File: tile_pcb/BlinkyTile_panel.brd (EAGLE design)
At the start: 220.1 x 170 mm, 210 parts

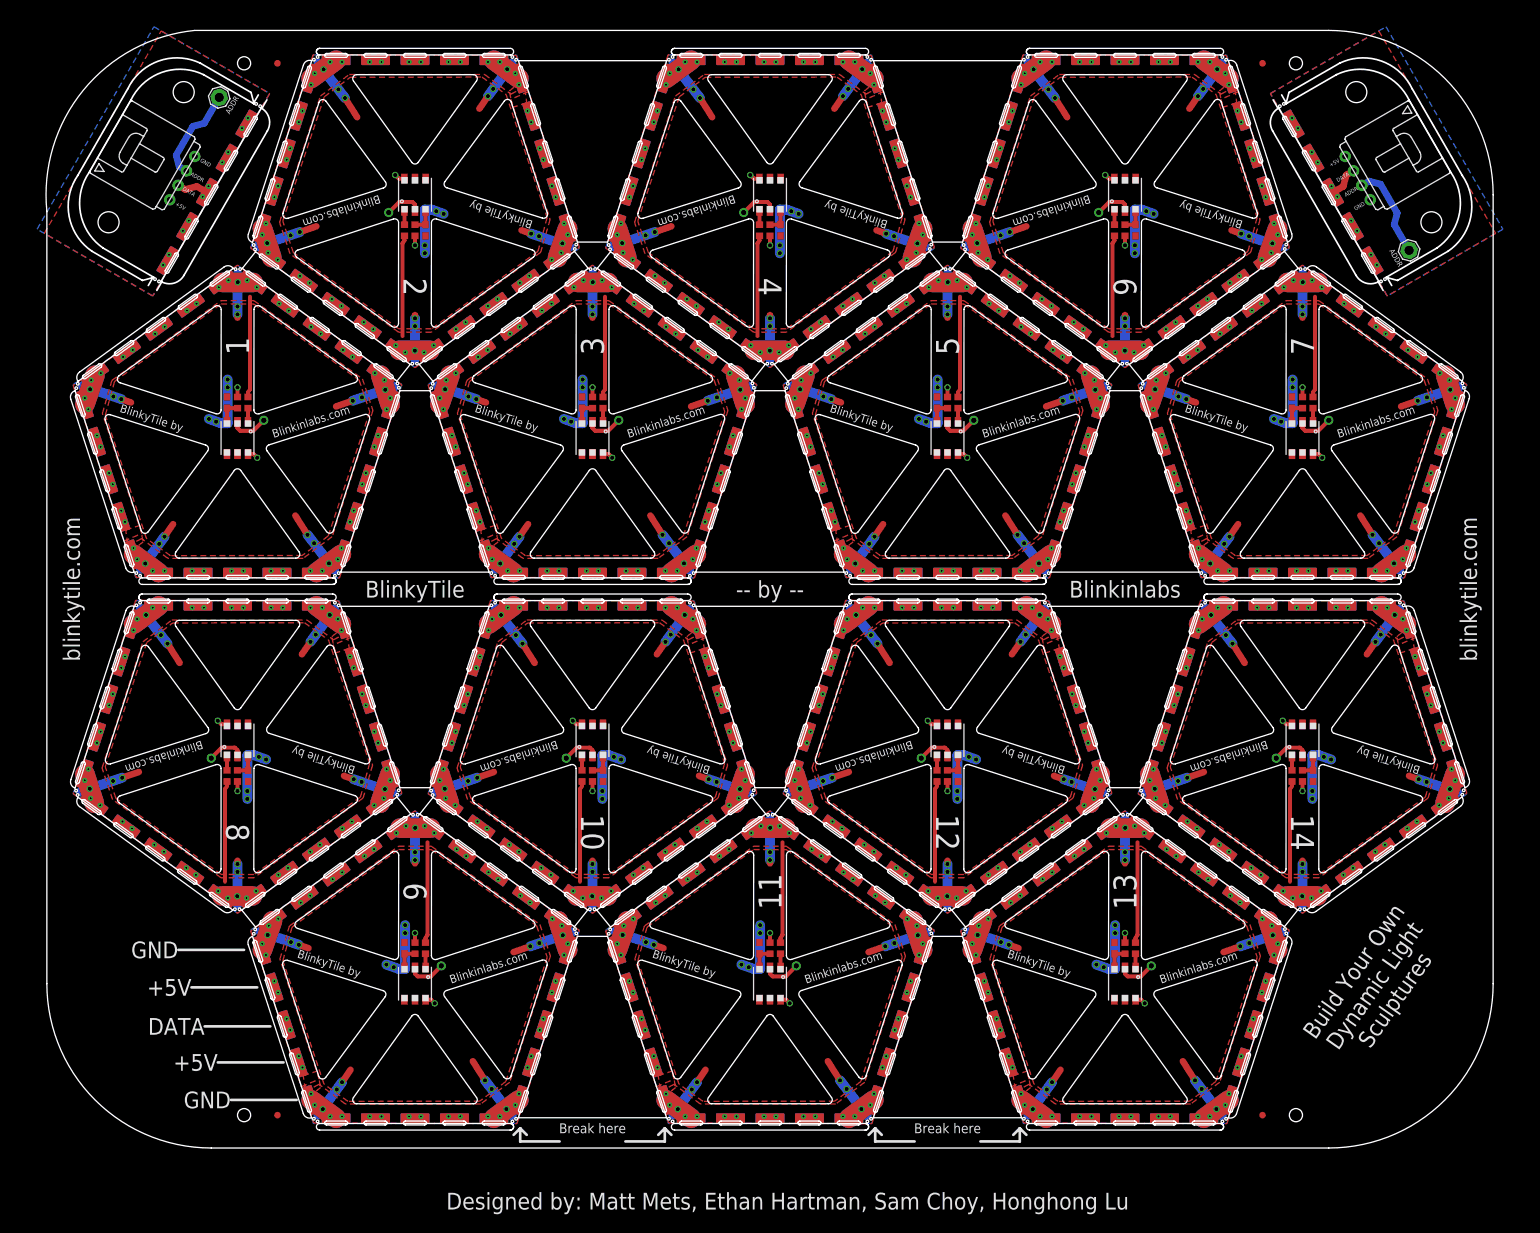
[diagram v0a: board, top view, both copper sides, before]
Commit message: Rev M panel from Sam
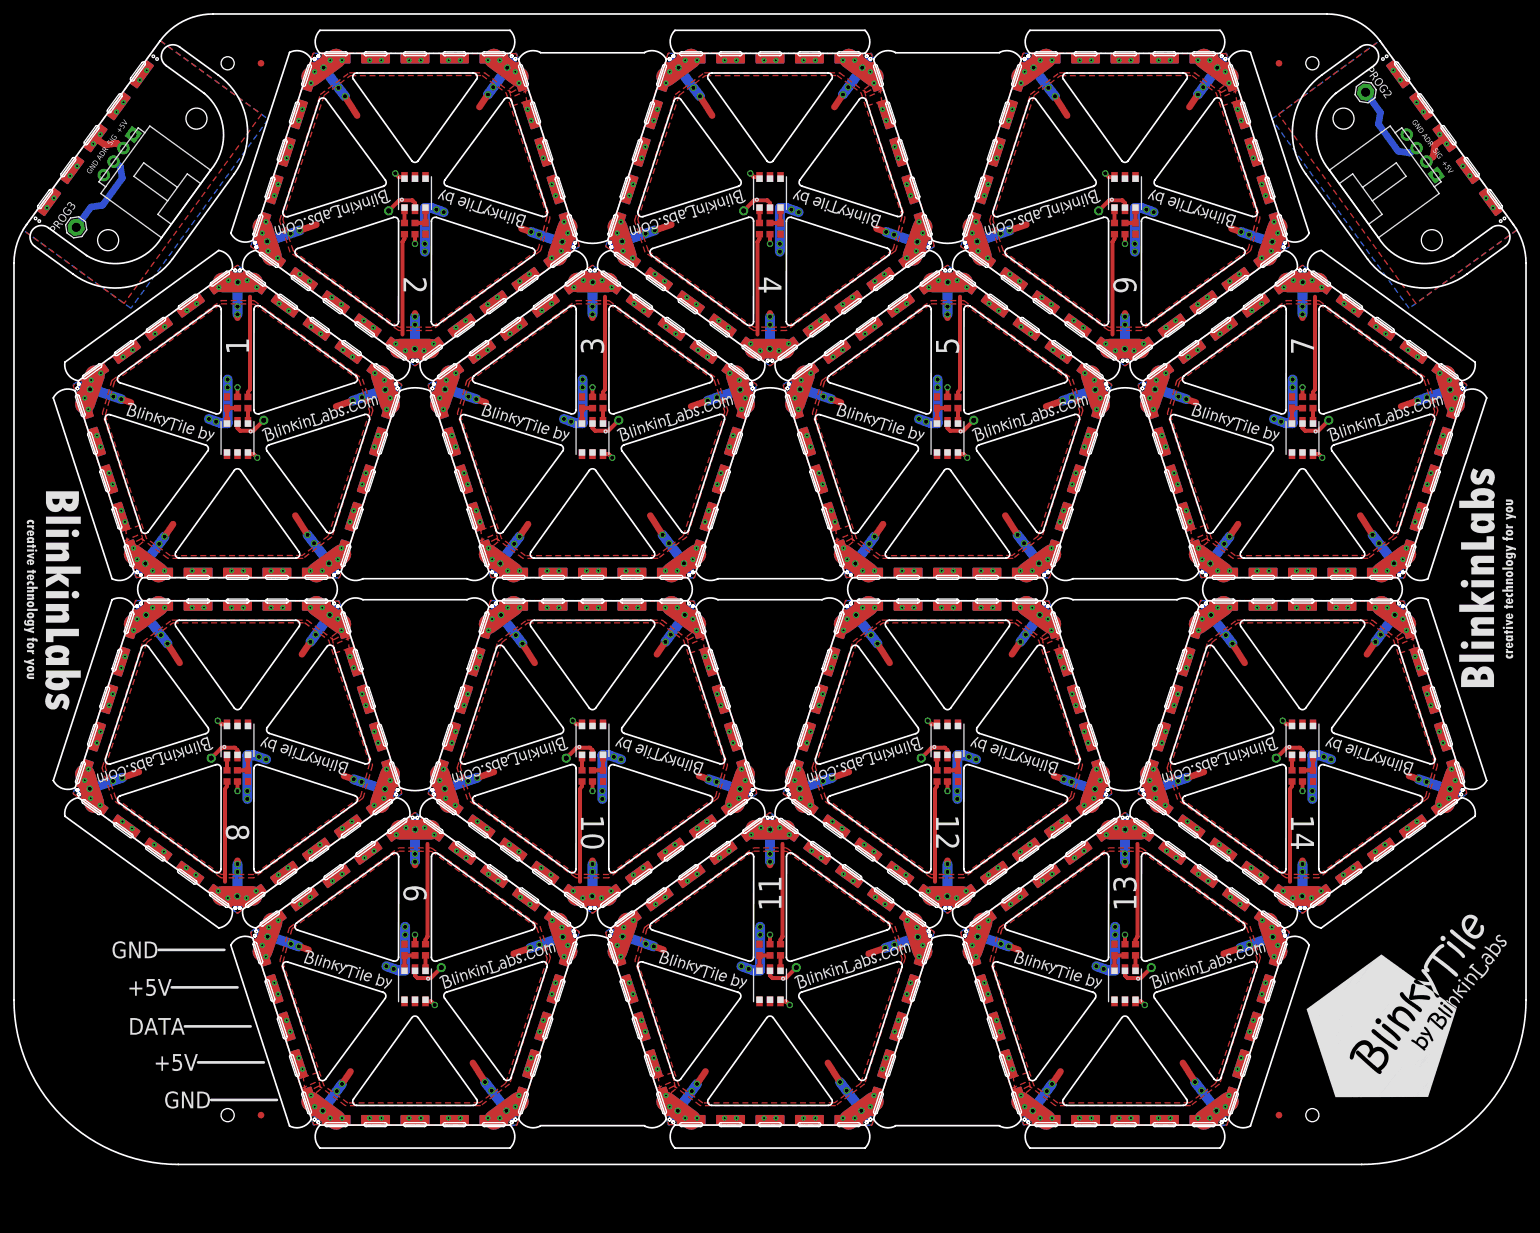
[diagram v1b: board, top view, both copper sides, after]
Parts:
- removed C1: .1uF, adafruit:C0603
- removed E$1, E$10, E$11, E$12, E$13, E$14, E$15, E$2, E$21, E$22, E$3, E$4, E$47, E$48, E$5, E$55, E$6, E$7, E$8, E$9: (no value), dodocohedreled:MOUSE_BITE_1
- removed E$16, E$17, E$19, E$20: (no value), dodocohedreled:MOUSE_BITE
- removed E$18: (no value), Sam-Lib:DUPONT-4P
- removed PROG, PROG1: (no value), solpad:SE14
- removed R1: 75, adafruit:R0603
- removed R2: 10k, adafruit:R0603
- removed U$2, U$3, U$4, U$5, U$6, U$91: D_EDGEMOD, dodocohedreled:D_EDGE_SLOT_MOD
- removed U$7: WS2822S_LED, blinkinlabs:WS2822S_LED
- added C4: .1uF, adafruit:C0603
- added E$100, E$101, E$102, E$103, E$104, E$105, E$106, E$107, E$108, E$109, E$110, E$111, E$112, E$113, E$114, E$115, E$116, E$117, E$118, E$119, E$120, E$121, E$122, E$123, E$124, E$125, E$126, E$127, E$128, E$129, E$130, E$131, E$132, E$133, E$134, E$135, E$136, E$137, E$138, E$139, E$140, E$141, E$142, E$143, E$144, E$145, E$146, E$147, E$148, E$149, E$150, E$151, E$152, E$153, E$154, E$155, E$156, E$157, E$158, E$159, E$160, E$161, E$162, E$163, E$164, E$165, E$166, E$167, E$168, E$169, E$170, E$171, E$172, E$173, E$174, E$175, E$176, E$177, E$178, E$179, E$180, E$181, E$182, E$183, E$184, E$185, E$186, E$187, E$188, E$189, E$190, E$191, E$192, E$193, E$199, E$200, E$202, E$203, E$81, E$82, E$83, E$84, E$85, E$86, E$87, E$88, E$89, E$90, E$91, E$92, E$93, E$94, E$95, E$96, E$97, E$98, E$99: (no value), dodocohedreled:MOUSE_BITE_1
- added E$201, E$204: (no value), dodocohedreled:4-PIN_DUPONT
- added E$205, E$206, E$207, E$208, E$209, E$210, E$211, E$212, E$213, E$214, E$215, E$216, E$217, E$218: (no value), dodocohedreled:BLINKYTILE
- added E$219: (no value), dodocohedreled:BLINKYTILELOGO
- added E$220, E$225: (no value), dodocohedreled:BLINKINLABSLOGO
- added E$221, E$222, E$223, E$224: (no value), SparkFun-Aesthetics:FIDUCIAL-1X2
- added PROG2, PROG3: (no value), solpad:SE14
- added R7: 75, adafruit:R0603
- added R8: 10k, adafruit:R0603
- added U$20, U$21, U$22, U$23, U$93, U$94: D_EDGEMOD, dodocohedreled:D_EDGE_SLOT_MOD
- added U$24: WS2822S_LED, blinkinlabs:WS2822S_LED
- E$76: device Sam-Lib:DUPONT-4P -> dodocohedreled:MOUSE_BITE_1
- E$77, E$78, E$79, E$80: device SparkFun-Aesthetics:FIDUCIAL-1X2 -> dodocohedreled:MOUSE_BITE_1
- moved E$67 207.0 mm to (105.3, 30.9), turned to 288 degrees
- moved E$80 202.4 mm to (78.3, 52.4), turned to 252 degrees
- moved E$70 188.5 mm to (81.0, 48.5), turned to 0 degrees
- moved E$73 184.2 mm to (81.0, 48.5), turned to 0 degrees
- moved U$44 182.5 mm to (-74.2, 66.8), turned to 252 degrees
- moved U$86 182.5 mm to (74.2, -66.8), turned to 72 degrees
- moved E$32 181.3 mm to (-105.3, 30.9), turned to 72 degrees
- moved E$72 174.3 mm to (105.3, 30.9), turned to 288 degrees
- moved E$78 164.8 mm to (39.0, 80.9), turned to 36 degrees
- moved U$46 160.0 mm to (-66.5, 43.0), turned to 324 degrees
- moved U$88 160.0 mm to (66.5, -43.0), turned to 144 degrees
- moved E$71 159.1 mm to (56.7, 30.9), turned to 72 degrees
- moved E$74 158.8 mm to (29.7, 52.4)
- moved U$43 156.7 mm to (-54.0, 81.5), turned to 180 degrees
- moved U$85 156.7 mm to (54.0, -81.5), turned to 0 degrees
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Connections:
- removed net 5V: R1.1, U$2.P$2, U$2.P$4, U$2.P$7, U$2.P$9, U$2.PWRVIA1, U$2.PWRVIA3, U$2.PWRVIA4, U$2.PWRVIA6, U$3.P$2, U$3.P$4, U$3.P$7, U$3.P$9, U$3.PWRVIA1, U$3.PWRVIA3, U$3.PWRVIA4, U$3.PWRVIA6, U$4.P$2, U$4.P$4, U$4.P$7, U$4.P$9, U$4.PWRVIA1, U$4.PWRVIA3, U$4.PWRVIA4, U$4.PWRVIA6, U$5.P$2, U$5.P$4, U$5.P$7, U$5.P$9, U$5.PWRVIA1, U$5.PWRVIA3, U$5.PWRVIA4, U$5.PWRVIA6, U$6.P$2, U$6.P$4, U$6.P$7, U$6.P$9, U$6.PWRVIA1, U$6.PWRVIA3, U$6.PWRVIA4, U$6.PWRVIA6, U$7.6
- removed net 5V1: R3.1, U$1.P$2, U$1.P$4, U$1.P$7, U$1.P$9, U$1.PWRVIA1, U$1.PWRVIA3, U$1.PWRVIA4, U$1.PWRVIA6, U$10.P$2, U$10.P$4, U$10.P$7, U$10.P$9, U$10.PWRVIA1, U$10.PWRVIA3, U$10.PWRVIA4, U$10.PWRVIA6, U$11.P$2, U$11.P$4, U$11.P$7, U$11.P$9, U$11.PWRVIA1, U$11.PWRVIA3, U$11.PWRVIA4, U$11.PWRVIA6, U$12.6, U$8.P$2, U$8.P$4, U$8.P$7, U$8.P$9, U$8.PWRVIA1, U$8.PWRVIA3, U$8.PWRVIA4, U$8.PWRVIA6, U$9.P$2, U$9.P$4, U$9.P$7, U$9.P$9, U$9.PWRVIA1, U$9.PWRVIA3, U$9.PWRVIA4, U$9.PWRVIA6
- removed net ADRI: U$7.2
- removed net DATA: R2.2, U$2.P$3, U$2.P$8, U$2.SIGVIA1, U$2.SIGVIA3, U$3.P$3, U$3.P$8, U$3.SIGVIA1, U$3.SIGVIA3, U$4.P$3, U$4.P$8, U$4.SIGVIA1, U$4.SIGVIA3, U$5.P$3, U$5.P$8, U$5.SIGVIA1, U$5.SIGVIA3, U$6.P$3, U$6.P$8, U$6.SIGVIA1, U$6.SIGVIA3
- removed net GND: C1.2, U$2.GNDVIA1, U$2.GNDVIA3, U$2.GNDVIA4, U$2.GNDVIA6, U$2.P$1, U$2.P$10, U$2.P$5, U$2.P$6, U$3.GNDVIA1, U$3.GNDVIA3, U$3.GNDVIA4, U$3.GNDVIA6, U$3.P$1, U$3.P$10, U$3.P$5, U$3.P$6, U$4.GNDVIA1, U$4.GNDVIA3, U$4.GNDVIA4, U$4.GNDVIA6, U$4.P$1, U$4.P$10, U$4.P$5, U$4.P$6, U$5.GNDVIA1, U$5.GNDVIA3, U$5.GNDVIA4, U$5.GNDVIA6, U$5.P$1, U$5.P$10, U$5.P$5, U$5.P$6, U$6.GNDVIA1, U$6.GNDVIA3, U$6.GNDVIA4, U$6.GNDVIA6, U$6.P$1, U$6.P$10, U$6.P$5, U$6.P$6, U$7.4
- removed net N$1: C1.1, R1.2, U$7.3
- removed net N$2: R2.1, U$7.1
- removed net S$1: E$18.P$2, U$91.P$3
- removed net S$10: E$18.P$3, PROG.MP
- removed net S$2: E$18.P$4, U$91.P$1, U$91.P$5
- removed net S$3: E$76.P$4, U$19.P$1, U$19.P$5
- removed net S$4: E$76.P$2, U$19.P$3
- removed net S$5: E$76.P$3, PROG1.MP
- removed net VCC: E$18.P$1, U$91.P$7, U$91.P$9
- removed net VCC1: E$76.P$1, U$19.P$7, U$19.P$9
- new net 5V15: R29.1, U$85.P$2, U$85.P$4, U$85.P$7, U$85.P$9, U$85.PWRVIA1, U$85.PWRVIA3, U$85.PWRVIA4, U$85.PWRVIA6, U$86.P$2, U$86.P$4, U$86.P$7, U$86.P$9, U$86.PWRVIA1, U$86.PWRVIA3, U$86.PWRVIA4, U$86.PWRVIA6, U$87.P$2, U$87.P$4, U$87.P$7, U$87.P$9, U$87.PWRVIA1, U$87.PWRVIA3, U$87.PWRVIA4, U$87.PWRVIA6, U$88.P$2, U$88.P$4, U$88.P$7, U$88.P$9, U$88.PWRVIA1, U$88.PWRVIA3, U$88.PWRVIA4, U$88.PWRVIA6, U$89.P$2, U$89.P$4, U$89.P$7, U$89.P$9, U$89.PWRVIA1, U$89.PWRVIA3, U$89.PWRVIA4, U$89.PWRVIA6, U$90.6
- new net 5V3: R5.1, U$13.P$2, U$13.P$4, U$13.P$7, U$13.P$9, U$13.PWRVIA1, U$13.PWRVIA3, U$13.PWRVIA4, U$13.PWRVIA6, U$14.P$2, U$14.P$4, U$14.P$7, U$14.P$9, U$14.PWRVIA1, U$14.PWRVIA3, U$14.PWRVIA4, U$14.PWRVIA6, U$15.P$2, U$15.P$4, U$15.P$7, U$15.P$9, U$15.PWRVIA1, U$15.PWRVIA3, U$15.PWRVIA4, U$15.PWRVIA6, U$16.P$2, U$16.P$4, U$16.P$7, U$16.P$9, U$16.PWRVIA1, U$16.PWRVIA3, U$16.PWRVIA4, U$16.PWRVIA6, U$17.P$2, U$17.P$4, U$17.P$7, U$17.P$9, U$17.PWRVIA1, U$17.PWRVIA3, U$17.PWRVIA4, U$17.PWRVIA6, U$18.6
- new net ADRI3: U$24.2
- new net DATA3: R8.2, U$19.P$3, U$19.P$8, U$19.SIGVIA1, U$19.SIGVIA3, U$20.P$3, U$20.P$8, U$20.SIGVIA1, U$20.SIGVIA3, U$21.P$3, U$21.P$8, U$21.SIGVIA1, U$21.SIGVIA3, U$22.P$3, U$22.P$8, U$22.SIGVIA1, U$22.SIGVIA3, U$23.P$3, U$23.P$8, U$23.SIGVIA1, U$23.SIGVIA3
- new net GND3: C4.2, U$19.GNDVIA1, U$19.GNDVIA3, U$19.GNDVIA4, U$19.GNDVIA6, U$19.P$1, U$19.P$10, U$19.P$5, U$19.P$6, U$20.GNDVIA1, U$20.GNDVIA3, U$20.GNDVIA4, U$20.GNDVIA6, U$20.P$1, U$20.P$10, U$20.P$5, U$20.P$6, U$21.GNDVIA1, U$21.GNDVIA3, U$21.GNDVIA4, U$21.GNDVIA6, U$21.P$1, U$21.P$10, U$21.P$5, U$21.P$6, U$22.GNDVIA1, U$22.GNDVIA3, U$22.GNDVIA4, U$22.GNDVIA6, U$22.P$1, U$22.P$10, U$22.P$5, U$22.P$6, U$23.GNDVIA1, U$23.GNDVIA3, U$23.GNDVIA4, U$23.GNDVIA6, U$23.P$1, U$23.P$10, U$23.P$5, U$23.P$6, U$24.4
- new net N$11: C4.1, R7.2, U$24.3
- new net N$12: R8.1, U$24.1
- new net S$11: E$204.P$2, U$94.P$3
- new net S$12: E$204.P$3, PROG3.MP
- new net S$6: E$201.P$4, U$93.P$1, U$93.P$5
- new net S$7: E$201.P$2, U$93.P$3
- new net S$8: E$201.P$3, PROG2.MP
- new net S$9: E$204.P$4, U$94.P$1, U$94.P$5
- new net VCC2: E$201.P$1, U$93.P$7, U$93.P$9
- new net VCC3: E$204.P$1, U$94.P$7, U$94.P$9
- net 5V10: now also R19.1, U$55.P$2, U$55.P$4, U$55.P$7, U$55.P$9, U$55.PWRVIA1, U$55.PWRVIA3, U$55.PWRVIA4, U$55.PWRVIA6, U$56.P$2, U$56.P$4, U$56.P$7, U$56.P$9, U$56.PWRVIA1, U$56.PWRVIA3, U$56.PWRVIA4, U$56.PWRVIA6, U$57.P$2, U$57.P$4, U$57.P$7, U$57.P$9, U$57.PWRVIA1, U$57.PWRVIA3, U$57.PWRVIA4, U$57.PWRVIA6, U$58.P$2, U$58.P$4, U$58.P$7, U$58.P$9, U$58.PWRVIA1, U$58.PWRVIA3, U$58.PWRVIA4, U$58.PWRVIA6, U$59.P$2, U$59.P$4, U$59.P$7, U$59.P$9, U$59.PWRVIA1, U$59.PWRVIA3, U$59.PWRVIA4, U$59.PWRVIA6, U$60.6; no longer R21.1, U$61.P$2, U$61.P$4, U$61.P$7, U$61.P$9, U$61.PWRVIA1, U$61.PWRVIA3, U$61.PWRVIA4, U$61.PWRVIA6, U$62.P$2, U$62.P$4, U$62.P$7, U$62.P$9, U$62.PWRVIA1, U$62.PWRVIA3, U$62.PWRVIA4, U$62.PWRVIA6, U$63.P$2, U$63.P$4, U$63.P$7, U$63.P$9, U$63.PWRVIA1, U$63.PWRVIA3, U$63.PWRVIA4, U$63.PWRVIA6, U$64.P$2, U$64.P$4, U$64.P$7, U$64.P$9, U$64.PWRVIA1, U$64.PWRVIA3, U$64.PWRVIA4, U$64.PWRVIA6, U$65.P$2, U$65.P$4, U$65.P$7, U$65.P$9, U$65.PWRVIA1, U$65.PWRVIA3, U$65.PWRVIA4, U$65.PWRVIA6, U$66.6
- net 5V11: now also R21.1, U$61.P$2, U$61.P$4, U$61.P$7, U$61.P$9, U$61.PWRVIA1, U$61.PWRVIA3, U$61.PWRVIA4, U$61.PWRVIA6, U$62.P$2, U$62.P$4, U$62.P$7, U$62.P$9, U$62.PWRVIA1, U$62.PWRVIA3, U$62.PWRVIA4, U$62.PWRVIA6, U$63.P$2, U$63.P$4, U$63.P$7, U$63.P$9, U$63.PWRVIA1, U$63.PWRVIA3, U$63.PWRVIA4, U$63.PWRVIA6, U$64.P$2, U$64.P$4, U$64.P$7, U$64.P$9, U$64.PWRVIA1, U$64.PWRVIA3, U$64.PWRVIA4, U$64.PWRVIA6, U$65.P$2, U$65.P$4, U$65.P$7, U$65.P$9, U$65.PWRVIA1, U$65.PWRVIA3, U$65.PWRVIA4, U$65.PWRVIA6, U$66.6; no longer R23.1, U$67.P$2, U$67.P$4, U$67.P$7, U$67.P$9, U$67.PWRVIA1, U$67.PWRVIA3, U$67.PWRVIA4, U$67.PWRVIA6, U$68.P$2, U$68.P$4, U$68.P$7, U$68.P$9, U$68.PWRVIA1, U$68.PWRVIA3, U$68.PWRVIA4, U$68.PWRVIA6, U$69.P$2, U$69.P$4, U$69.P$7, U$69.P$9, U$69.PWRVIA1, U$69.PWRVIA3, U$69.PWRVIA4, U$69.PWRVIA6, U$70.P$2, U$70.P$4, U$70.P$7, U$70.P$9, U$70.PWRVIA1, U$70.PWRVIA3, U$70.PWRVIA4, U$70.PWRVIA6, U$71.P$2, U$71.P$4, U$71.P$7, U$71.P$9, U$71.PWRVIA1, U$71.PWRVIA3, U$71.PWRVIA4, U$71.PWRVIA6, U$72.6
- net 5V12: now also R23.1, U$67.P$2, U$67.P$4, U$67.P$7, U$67.P$9, U$67.PWRVIA1, U$67.PWRVIA3, U$67.PWRVIA4, U$67.PWRVIA6, U$68.P$2, U$68.P$4, U$68.P$7, U$68.P$9, U$68.PWRVIA1, U$68.PWRVIA3, U$68.PWRVIA4, U$68.PWRVIA6, U$69.P$2, U$69.P$4, U$69.P$7, U$69.P$9, U$69.PWRVIA1, U$69.PWRVIA3, U$69.PWRVIA4, U$69.PWRVIA6, U$70.P$2, U$70.P$4, U$70.P$7, U$70.P$9, U$70.PWRVIA1, U$70.PWRVIA3, U$70.PWRVIA4, U$70.PWRVIA6, U$71.P$2, U$71.P$4, U$71.P$7, U$71.P$9, U$71.PWRVIA1, U$71.PWRVIA3, U$71.PWRVIA4, U$71.PWRVIA6, U$72.6; no longer R25.1, U$73.P$2, U$73.P$4, U$73.P$7, U$73.P$9, U$73.PWRVIA1, U$73.PWRVIA3, U$73.PWRVIA4, U$73.PWRVIA6, U$74.P$2, U$74.P$4, U$74.P$7, U$74.P$9, U$74.PWRVIA1, U$74.PWRVIA3, U$74.PWRVIA4, U$74.PWRVIA6, U$75.P$2, U$75.P$4, U$75.P$7, U$75.P$9, U$75.PWRVIA1, U$75.PWRVIA3, U$75.PWRVIA4, U$75.PWRVIA6, U$76.P$2, U$76.P$4, U$76.P$7, U$76.P$9, U$76.PWRVIA1, U$76.PWRVIA3, U$76.PWRVIA4, U$76.PWRVIA6, U$77.P$2, U$77.P$4, U$77.P$7, U$77.P$9, U$77.PWRVIA1, U$77.PWRVIA3, U$77.PWRVIA4, U$77.PWRVIA6, U$78.6
- net 5V13: now also R25.1, U$73.P$2, U$73.P$4, U$73.P$7, U$73.P$9, U$73.PWRVIA1, U$73.PWRVIA3, U$73.PWRVIA4, U$73.PWRVIA6, U$74.P$2, U$74.P$4, U$74.P$7, U$74.P$9, U$74.PWRVIA1, U$74.PWRVIA3, U$74.PWRVIA4, U$74.PWRVIA6, U$75.P$2, U$75.P$4, U$75.P$7, U$75.P$9, U$75.PWRVIA1, U$75.PWRVIA3, U$75.PWRVIA4, U$75.PWRVIA6, U$76.P$2, U$76.P$4, U$76.P$7, U$76.P$9, U$76.PWRVIA1, U$76.PWRVIA3, U$76.PWRVIA4, U$76.PWRVIA6, U$77.P$2, U$77.P$4, U$77.P$7, U$77.P$9, U$77.PWRVIA1, U$77.PWRVIA3, U$77.PWRVIA4, U$77.PWRVIA6, U$78.6; no longer R27.1, U$79.P$2, U$79.P$4, U$79.P$7, U$79.P$9, U$79.PWRVIA1, U$79.PWRVIA3, U$79.PWRVIA4, U$79.PWRVIA6, U$80.P$2, U$80.P$4, U$80.P$7, U$80.P$9, U$80.PWRVIA1, U$80.PWRVIA3, U$80.PWRVIA4, U$80.PWRVIA6, U$81.P$2, U$81.P$4, U$81.P$7, U$81.P$9, U$81.PWRVIA1, U$81.PWRVIA3, U$81.PWRVIA4, U$81.PWRVIA6, U$82.P$2, U$82.P$4, U$82.P$7, U$82.P$9, U$82.PWRVIA1, U$82.PWRVIA3, U$82.PWRVIA4, U$82.PWRVIA6, U$83.P$2, U$83.P$4, U$83.P$7, U$83.P$9, U$83.PWRVIA1, U$83.PWRVIA3, U$83.PWRVIA4, U$83.PWRVIA6, U$84.6
- net 5V14: now also R27.1, U$79.P$2, U$79.P$4, U$79.P$7, U$79.P$9, U$79.PWRVIA1, U$79.PWRVIA3, U$79.PWRVIA4, U$79.PWRVIA6, U$80.P$2, U$80.P$4, U$80.P$7, U$80.P$9, U$80.PWRVIA1, U$80.PWRVIA3, U$80.PWRVIA4, U$80.PWRVIA6, U$81.P$2, U$81.P$4, U$81.P$7, U$81.P$9, U$81.PWRVIA1, U$81.PWRVIA3, U$81.PWRVIA4, U$81.PWRVIA6, U$82.P$2, U$82.P$4, U$82.P$7, U$82.P$9, U$82.PWRVIA1, U$82.PWRVIA3, U$82.PWRVIA4, U$82.PWRVIA6, U$83.P$2, U$83.P$4, U$83.P$7, U$83.P$9, U$83.PWRVIA1, U$83.PWRVIA3, U$83.PWRVIA4, U$83.PWRVIA6, U$84.6; no longer R29.1, U$85.P$2, U$85.P$4, U$85.P$7, U$85.P$9, U$85.PWRVIA1, U$85.PWRVIA3, U$85.PWRVIA4, U$85.PWRVIA6, U$86.P$2, U$86.P$4, U$86.P$7, U$86.P$9, U$86.PWRVIA1, U$86.PWRVIA3, U$86.PWRVIA4, U$86.PWRVIA6, U$87.P$2, U$87.P$4, U$87.P$7, U$87.P$9, U$87.PWRVIA1, U$87.PWRVIA3, U$87.PWRVIA4, U$87.PWRVIA6, U$88.P$2, U$88.P$4, U$88.P$7, U$88.P$9, U$88.PWRVIA1, U$88.PWRVIA3, U$88.PWRVIA4, U$88.PWRVIA6, U$89.P$2, U$89.P$4, U$89.P$7, U$89.P$9, U$89.PWRVIA1, U$89.PWRVIA3, U$89.PWRVIA4, U$89.PWRVIA6, U$90.6
- net 5V2: now also R3.1, U$1.P$2, U$1.P$4, U$1.P$7, U$1.P$9, U$1.PWRVIA1, U$1.PWRVIA3, U$1.PWRVIA4, U$1.PWRVIA6, U$10.P$2, U$10.P$4, U$10.P$7, U$10.P$9, U$10.PWRVIA1, U$10.PWRVIA3, U$10.PWRVIA4, U$10.PWRVIA6, U$11.P$2, U$11.P$4, U$11.P$7, U$11.P$9, U$11.PWRVIA1, U$11.PWRVIA3, U$11.PWRVIA4, U$11.PWRVIA6, U$12.6, U$8.P$2, U$8.P$4, U$8.P$7, U$8.P$9, U$8.PWRVIA1, U$8.PWRVIA3, U$8.PWRVIA4, U$8.PWRVIA6, U$9.P$2, U$9.P$4, U$9.P$7, U$9.P$9, U$9.PWRVIA1, U$9.PWRVIA3, U$9.PWRVIA4, U$9.PWRVIA6; no longer R5.1, U$13.P$2, U$13.P$4, U$13.P$7, U$13.P$9, U$13.PWRVIA1, U$13.PWRVIA3, U$13.PWRVIA4, U$13.PWRVIA6, U$14.P$2, U$14.P$4, U$14.P$7, U$14.P$9, U$14.PWRVIA1, U$14.PWRVIA3, U$14.PWRVIA4, U$14.PWRVIA6, U$15.P$2, U$15.P$4, U$15.P$7, U$15.P$9, U$15.PWRVIA1, U$15.PWRVIA3, U$15.PWRVIA4, U$15.PWRVIA6, U$16.P$2, U$16.P$4, U$16.P$7, U$16.P$9, U$16.PWRVIA1, U$16.PWRVIA3, U$16.PWRVIA4, U$16.PWRVIA6, U$17.P$2, U$17.P$4, U$17.P$7, U$17.P$9, U$17.PWRVIA1, U$17.PWRVIA3, U$17.PWRVIA4, U$17.PWRVIA6, U$18.6
- net 5V4: now also R7.1, U$19.P$2, U$19.P$4, U$19.P$7, U$19.P$9, U$19.PWRVIA1, U$19.PWRVIA3, U$19.PWRVIA4, U$19.PWRVIA6, U$20.P$2, U$20.P$4, U$20.P$7, U$20.P$9, U$20.PWRVIA1, U$20.PWRVIA3, U$20.PWRVIA4, U$20.PWRVIA6, U$21.P$2, U$21.P$4, U$21.P$7, U$21.P$9, U$21.PWRVIA1, U$21.PWRVIA3, U$21.PWRVIA4, U$21.PWRVIA6, U$22.P$2, U$22.P$4, U$22.P$7, U$22.P$9, U$22.PWRVIA1, U$22.PWRVIA3, U$22.PWRVIA4, U$22.PWRVIA6, U$23.P$2, U$23.P$4, U$23.P$7, U$23.P$9, U$23.PWRVIA1, U$23.PWRVIA3, U$23.PWRVIA4, U$23.PWRVIA6, U$24.6; no longer R9.1, U$25.P$2, U$25.P$4, U$25.P$7, U$25.P$9, U$25.PWRVIA1, U$25.PWRVIA3, U$25.PWRVIA4, U$25.PWRVIA6, U$26.P$2, U$26.P$4, U$26.P$7, U$26.P$9, U$26.PWRVIA1, U$26.PWRVIA3, U$26.PWRVIA4, U$26.PWRVIA6, U$27.P$2, U$27.P$4, U$27.P$7, U$27.P$9, U$27.PWRVIA1, U$27.PWRVIA3, U$27.PWRVIA4, U$27.PWRVIA6, U$28.P$2, U$28.P$4, U$28.P$7, U$28.P$9, U$28.PWRVIA1, U$28.PWRVIA3, U$28.PWRVIA4, U$28.PWRVIA6, U$29.P$2, U$29.P$4, U$29.P$7, U$29.P$9, U$29.PWRVIA1, U$29.PWRVIA3, U$29.PWRVIA4, U$29.PWRVIA6, U$30.6
- net 5V5: now also R9.1, U$25.P$2, U$25.P$4, U$25.P$7, U$25.P$9, U$25.PWRVIA1, U$25.PWRVIA3, U$25.PWRVIA4, U$25.PWRVIA6, U$26.P$2, U$26.P$4, U$26.P$7, U$26.P$9, U$26.PWRVIA1, U$26.PWRVIA3, U$26.PWRVIA4, U$26.PWRVIA6, U$27.P$2, U$27.P$4, U$27.P$7, U$27.P$9, U$27.PWRVIA1, U$27.PWRVIA3, U$27.PWRVIA4, U$27.PWRVIA6, U$28.P$2, U$28.P$4, U$28.P$7, U$28.P$9, U$28.PWRVIA1, U$28.PWRVIA3, U$28.PWRVIA4, U$28.PWRVIA6, U$29.P$2, U$29.P$4, U$29.P$7, U$29.P$9, U$29.PWRVIA1, U$29.PWRVIA3, U$29.PWRVIA4, U$29.PWRVIA6, U$30.6; no longer R11.1, U$31.P$2, U$31.P$4, U$31.P$7, U$31.P$9, U$31.PWRVIA1, U$31.PWRVIA3, U$31.PWRVIA4, U$31.PWRVIA6, U$32.P$2, U$32.P$4, U$32.P$7, U$32.P$9, U$32.PWRVIA1, U$32.PWRVIA3, U$32.PWRVIA4, U$32.PWRVIA6, U$33.P$2, U$33.P$4, U$33.P$7, U$33.P$9, U$33.PWRVIA1, U$33.PWRVIA3, U$33.PWRVIA4, U$33.PWRVIA6, U$34.P$2, U$34.P$4, U$34.P$7, U$34.P$9, U$34.PWRVIA1, U$34.PWRVIA3, U$34.PWRVIA4, U$34.PWRVIA6, U$35.P$2, U$35.P$4, U$35.P$7, U$35.P$9, U$35.PWRVIA1, U$35.PWRVIA3, U$35.PWRVIA4, U$35.PWRVIA6, U$36.6
- net 5V6: now also R11.1, U$31.P$2, U$31.P$4, U$31.P$7, U$31.P$9, U$31.PWRVIA1, U$31.PWRVIA3, U$31.PWRVIA4, U$31.PWRVIA6, U$32.P$2, U$32.P$4, U$32.P$7, U$32.P$9, U$32.PWRVIA1, U$32.PWRVIA3, U$32.PWRVIA4, U$32.PWRVIA6, U$33.P$2, U$33.P$4, U$33.P$7, U$33.P$9, U$33.PWRVIA1, U$33.PWRVIA3, U$33.PWRVIA4, U$33.PWRVIA6, U$34.P$2, U$34.P$4, U$34.P$7, U$34.P$9, U$34.PWRVIA1, U$34.PWRVIA3, U$34.PWRVIA4, U$34.PWRVIA6, U$35.P$2, U$35.P$4, U$35.P$7, U$35.P$9, U$35.PWRVIA1, U$35.PWRVIA3, U$35.PWRVIA4, U$35.PWRVIA6, U$36.6; no longer R13.1, U$37.P$2, U$37.P$4, U$37.P$7, U$37.P$9, U$37.PWRVIA1, U$37.PWRVIA3, U$37.PWRVIA4, U$37.PWRVIA6, U$38.P$2, U$38.P$4, U$38.P$7, U$38.P$9, U$38.PWRVIA1, U$38.PWRVIA3, U$38.PWRVIA4, U$38.PWRVIA6, U$39.P$2, U$39.P$4, U$39.P$7, U$39.P$9, U$39.PWRVIA1, U$39.PWRVIA3, U$39.PWRVIA4, U$39.PWRVIA6, U$40.P$2, U$40.P$4, U$40.P$7, U$40.P$9, U$40.PWRVIA1, U$40.PWRVIA3, U$40.PWRVIA4, U$40.PWRVIA6, U$41.P$2, U$41.P$4, U$41.P$7, U$41.P$9, U$41.PWRVIA1, U$41.PWRVIA3, U$41.PWRVIA4, U$41.PWRVIA6, U$42.6
- net 5V7: now also R13.1, U$37.P$2, U$37.P$4, U$37.P$7, U$37.P$9, U$37.PWRVIA1, U$37.PWRVIA3, U$37.PWRVIA4, U$37.PWRVIA6, U$38.P$2, U$38.P$4, U$38.P$7, U$38.P$9, U$38.PWRVIA1, U$38.PWRVIA3, U$38.PWRVIA4, U$38.PWRVIA6, U$39.P$2, U$39.P$4, U$39.P$7, U$39.P$9, U$39.PWRVIA1, U$39.PWRVIA3, U$39.PWRVIA4, U$39.PWRVIA6, U$40.P$2, U$40.P$4, U$40.P$7, U$40.P$9, U$40.PWRVIA1, U$40.PWRVIA3, U$40.PWRVIA4, U$40.PWRVIA6, U$41.P$2, U$41.P$4, U$41.P$7, U$41.P$9, U$41.PWRVIA1, U$41.PWRVIA3, U$41.PWRVIA4, U$41.PWRVIA6, U$42.6; no longer R15.1, U$43.P$2, U$43.P$4, U$43.P$7, U$43.P$9, U$43.PWRVIA1, U$43.PWRVIA3, U$43.PWRVIA4, U$43.PWRVIA6, U$44.P$2, U$44.P$4, U$44.P$7, U$44.P$9, U$44.PWRVIA1, U$44.PWRVIA3, U$44.PWRVIA4, U$44.PWRVIA6, U$45.P$2, U$45.P$4, U$45.P$7, U$45.P$9, U$45.PWRVIA1, U$45.PWRVIA3, U$45.PWRVIA4, U$45.PWRVIA6, U$46.P$2, U$46.P$4, U$46.P$7, U$46.P$9, U$46.PWRVIA1, U$46.PWRVIA3, U$46.PWRVIA4, U$46.PWRVIA6, U$47.P$2, U$47.P$4, U$47.P$7, U$47.P$9, U$47.PWRVIA1, U$47.PWRVIA3, U$47.PWRVIA4, U$47.PWRVIA6, U$48.6
- net 5V8: now also R15.1, U$43.P$2, U$43.P$4, U$43.P$7, U$43.P$9, U$43.PWRVIA1, U$43.PWRVIA3, U$43.PWRVIA4, U$43.PWRVIA6, U$44.P$2, U$44.P$4, U$44.P$7, U$44.P$9, U$44.PWRVIA1, U$44.PWRVIA3, U$44.PWRVIA4, U$44.PWRVIA6, U$45.P$2, U$45.P$4, U$45.P$7, U$45.P$9, U$45.PWRVIA1, U$45.PWRVIA3, U$45.PWRVIA4, U$45.PWRVIA6, U$46.P$2, U$46.P$4, U$46.P$7, U$46.P$9, U$46.PWRVIA1, U$46.PWRVIA3, U$46.PWRVIA4, U$46.PWRVIA6, U$47.P$2, U$47.P$4, U$47.P$7, U$47.P$9, U$47.PWRVIA1, U$47.PWRVIA3, U$47.PWRVIA4, U$47.PWRVIA6, U$48.6; no longer R17.1, U$49.P$2, U$49.P$4, U$49.P$7, U$49.P$9, U$49.PWRVIA1, U$49.PWRVIA3, U$49.PWRVIA4, U$49.PWRVIA6, U$50.P$2, U$50.P$4, U$50.P$7, U$50.P$9, U$50.PWRVIA1, U$50.PWRVIA3, U$50.PWRVIA4, U$50.PWRVIA6, U$51.P$2, U$51.P$4, U$51.P$7, U$51.P$9, U$51.PWRVIA1, U$51.PWRVIA3, U$51.PWRVIA4, U$51.PWRVIA6, U$52.P$2, U$52.P$4, U$52.P$7, U$52.P$9, U$52.PWRVIA1, U$52.PWRVIA3, U$52.PWRVIA4, U$52.PWRVIA6, U$53.P$2, U$53.P$4, U$53.P$7, U$53.P$9, U$53.PWRVIA1, U$53.PWRVIA3, U$53.PWRVIA4, U$53.PWRVIA6, U$54.6
- net 5V9: now also R17.1, U$49.P$2, U$49.P$4, U$49.P$7, U$49.P$9, U$49.PWRVIA1, U$49.PWRVIA3, U$49.PWRVIA4, U$49.PWRVIA6, U$50.P$2, U$50.P$4, U$50.P$7, U$50.P$9, U$50.PWRVIA1, U$50.PWRVIA3, U$50.PWRVIA4, U$50.PWRVIA6, U$51.P$2, U$51.P$4, U$51.P$7, U$51.P$9, U$51.PWRVIA1, U$51.PWRVIA3, U$51.PWRVIA4, U$51.PWRVIA6, U$52.P$2, U$52.P$4, U$52.P$7, U$52.P$9, U$52.PWRVIA1, U$52.PWRVIA3, U$52.PWRVIA4, U$52.PWRVIA6, U$53.P$2, U$53.P$4, U$53.P$7, U$53.P$9, U$53.PWRVIA1, U$53.PWRVIA3, U$53.PWRVIA4, U$53.PWRVIA6, U$54.6; no longer R19.1, U$55.P$2, U$55.P$4, U$55.P$7, U$55.P$9, U$55.PWRVIA1, U$55.PWRVIA3, U$55.PWRVIA4, U$55.PWRVIA6, U$56.P$2, U$56.P$4, U$56.P$7, U$56.P$9, U$56.PWRVIA1, U$56.PWRVIA3, U$56.PWRVIA4, U$56.PWRVIA6, U$57.P$2, U$57.P$4, U$57.P$7, U$57.P$9, U$57.PWRVIA1, U$57.PWRVIA3, U$57.PWRVIA4, U$57.PWRVIA6, U$58.P$2, U$58.P$4, U$58.P$7, U$58.P$9, U$58.PWRVIA1, U$58.PWRVIA3, U$58.PWRVIA4, U$58.PWRVIA6, U$59.P$2, U$59.P$4, U$59.P$7, U$59.P$9, U$59.PWRVIA1, U$59.PWRVIA3, U$59.PWRVIA4, U$59.PWRVIA6, U$60.6
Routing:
- net GND3: track 0.00 -> 111.7 mm, vias 0 -> 19
- net GND: track 111.7 -> 0.00 mm, vias 19 -> 0
- net DATA: track 15.3 -> 0.00 mm
- net DATA3: track 0.00 -> 15.3 mm
- net S$10: track 14.5 -> 0.00 mm
- net S$5: track 14.5 -> 0.00 mm
- net S$8: track 0.00 -> 13.8 mm
- net S$12: track 0.00 -> 13.8 mm
- net ADRI3: track 0.00 -> 5.78 mm, vias 0 -> 1
- net ADRI: track 5.78 -> 0.00 mm, vias 1 -> 0
- net S$11: track 0.00 -> 4.88 mm
- net S$7: track 0.00 -> 4.88 mm
- net S$1: track 4.88 -> 0.00 mm
- net S$4: track 4.88 -> 0.00 mm
- net N$11: track 0.00 -> 3.70 mm
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- added copper zone on layer 16, net 5V15
- added copper zone on layer 16, net 5V3
- added copper zone on layer 1, net DATA3
- added copper zone on layer 1, net GND3
- added copper zone on layer 1, net N$10
- added copper zone on layer 1, net S$6
- added copper zone on layer 1, net S$9
- added copper zone on layer 16, net VCC2
- added copper zone on layer 16, net VCC3
- removed copper zone on layer 16, net 5V
- removed copper zone on layer 16, net 5V1
- removed copper zone on layer 1, net DATA
- removed copper zone on layer 1, net GND
- removed copper zone on layer 1, net N$4
- removed copper zone on layer 1, net S$2
- removed copper zone on layer 1, net S$3
- removed copper zone on layer 16, net VCC
- removed copper zone on layer 16, net VCC1
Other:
- board size 220.1 x 170 mm -> 230 x 175 mm
- board text added: "ADR"
- board text added: "SIG"
- board text removed: "-- by --"
- board text removed: "ADDR"
- board text removed: "ADDRESS"
- board text removed: "Blinkinlabs"
- board text removed: "Blinkinlabs.com"
- board text removed: "BlinkyTile"
- board text removed: "BlinkyTile by"
- board text removed: "Break here"
- board text removed: "Build Your Own Dynamic Light Sculptures"
- board text removed: "Designed by: Matt Mets, Ethan Hartman, Sam Choy, Honghong Lu"
- board text removed: "blinkytile.com"
